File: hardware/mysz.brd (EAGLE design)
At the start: 144.8 x 102.5 mm, 30 parts, among them IC1 LM1117T(H)-3.3, IC2 LM1117T(H)-3.3, U1 NUCLEO-L053R8

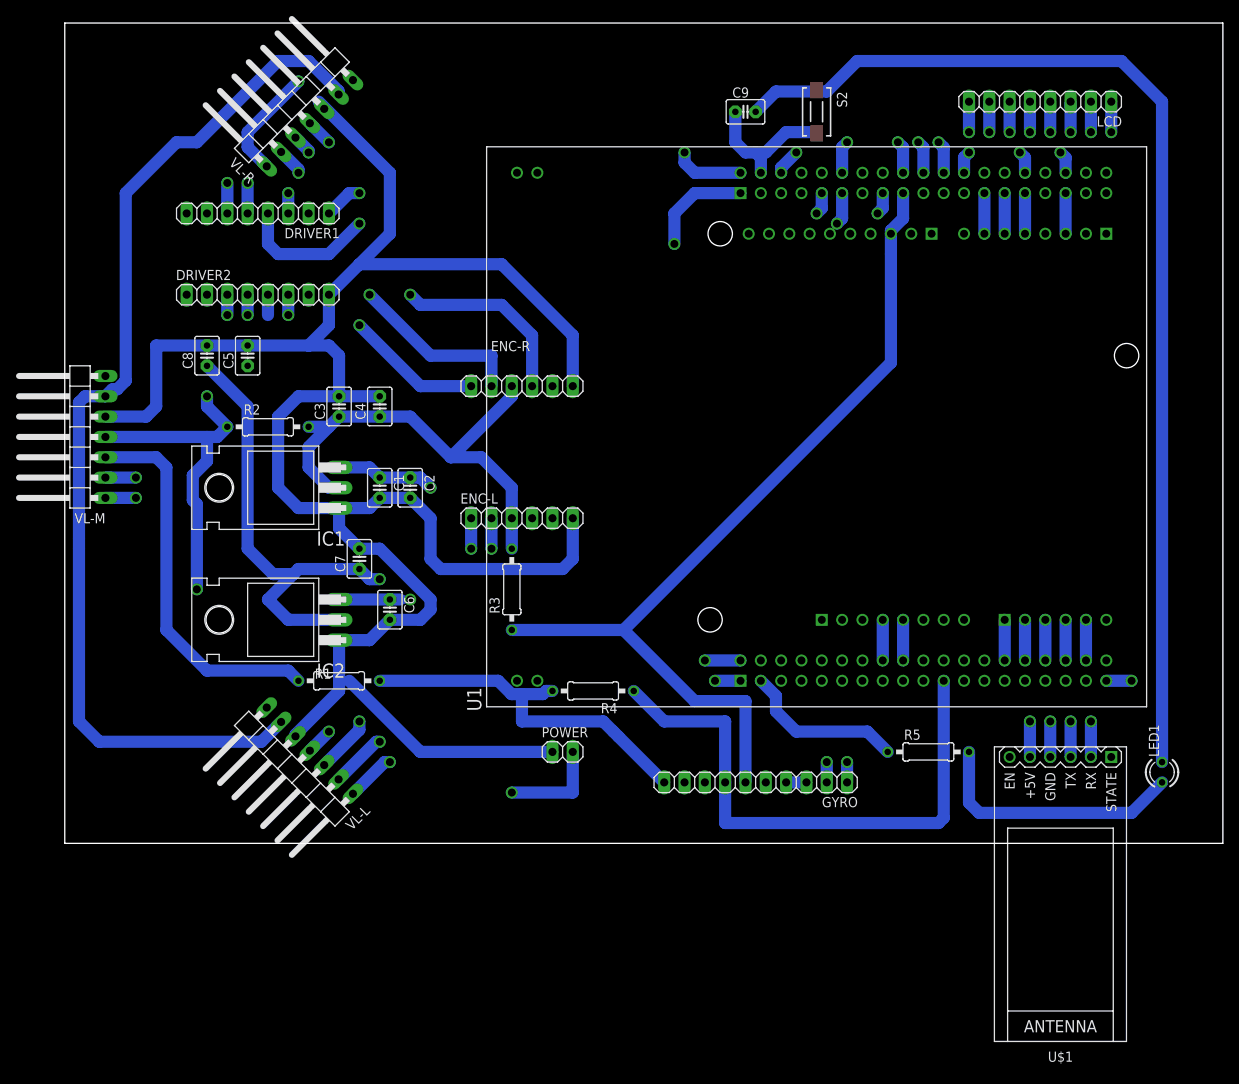
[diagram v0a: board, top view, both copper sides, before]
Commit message: Updated dim.brd
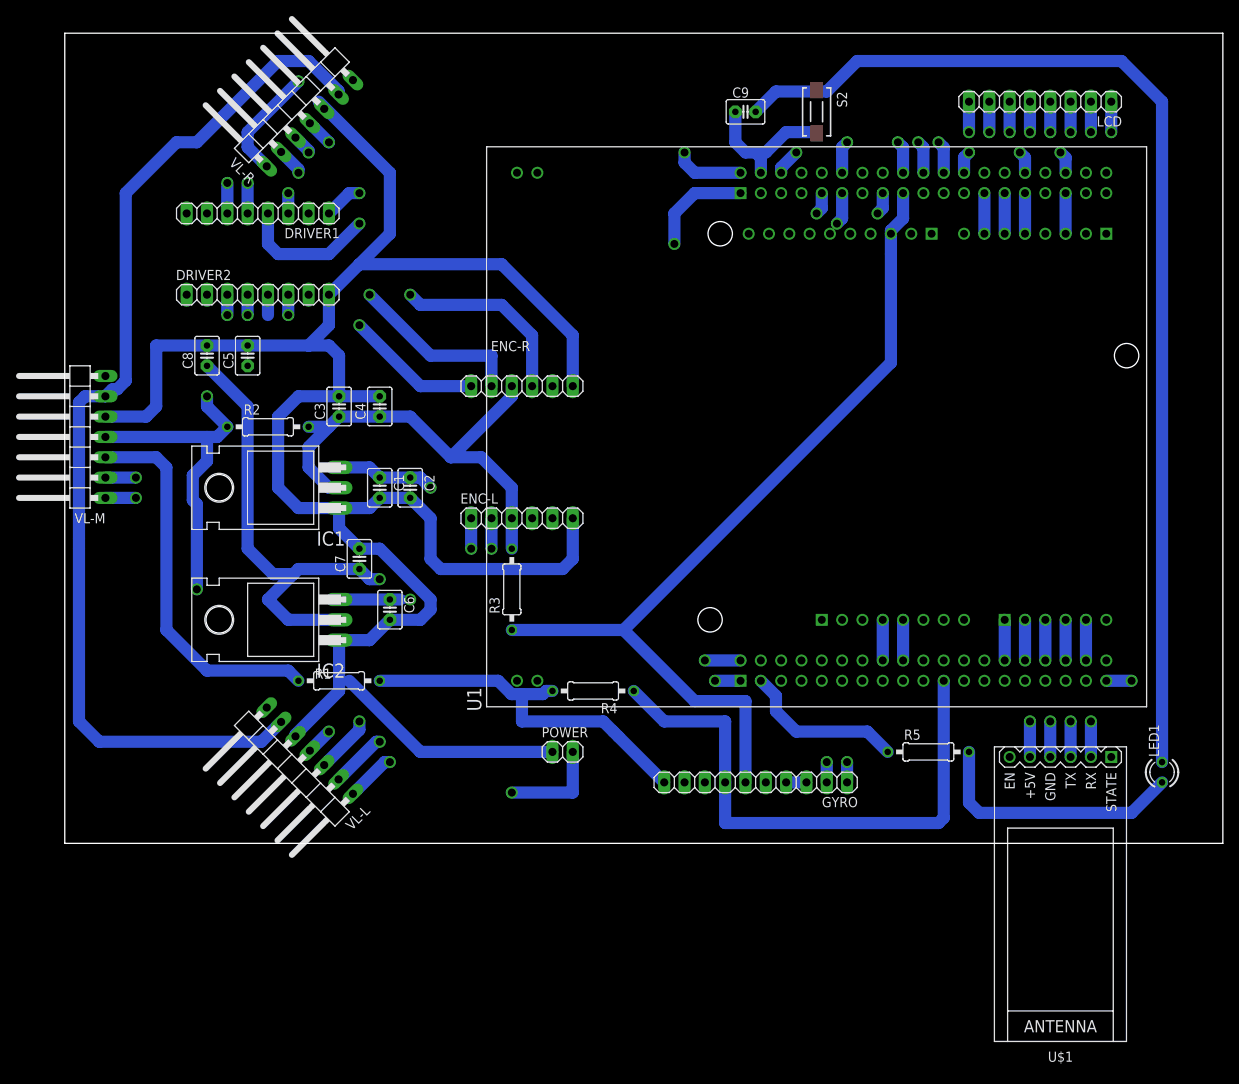
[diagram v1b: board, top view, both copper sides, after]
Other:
- board size 144.8 x 102.5 mm -> 144.8 x 101.3 mm
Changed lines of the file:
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@@
 <plain>
 <wire x1="0" y1="0" x2="144.76" y2="0" width="0" layer="20"/>
-<wire x1="144.76" y1="0" x2="144.76" y2="102.54" width="0" layer="20"/>
-<wire x1="144.76" y1="102.54" x2="0" y2="102.54" width="0" layer="20"/>
-<wire x1="0" y1="102.54" x2="0" y2="0" width="0" layer="20"/>
+<wire x1="144.76" y1="0" x2="144.76" y2="101.27" width="0" layer="20"/>
+<wire x1="144.76" y1="101.27" x2="0" y2="101.27" width="0" layer="20"/>
+<wire x1="0" y1="101.27" x2="0" y2="0" width="0" layer="20"/>
 <dimension x1="-3.81" y1="0" x2="-3.81" y2="100.33" x3="-11.43" y3="50.165" textsize="1.778" layer="1" dtype="horizontal"/>
 <dimension x1="-6.35" y1="0" x2="-6.35" y2="49.53" x3="-6.35" y3="49.53" textsize="1.778" layer="1" dtype="diameter"/>
 <dimension x1="-6.35" y1="49.53" x2="-6.35" y2="100.33" x3="-6.35" y3="100.33" textsize="1.778" layer="1" dtype="diameter"/>
-<dimension x1="64.77" y1="87.63" x2="148.59" y2="87.63" x3="106.68" y3="101.6" textsize="1.778" layer="1"/>
+<dimension x1="0" y1="101.27" x2="144.78" y2="101.6" x3="72.39" y3="111.76" textsize="1.778" layer="1" dtype="horizontal"/>
+<dimension x1="134.62" y1="77.47" x2="53.34" y2="77.47" x3="93.98" y3="105.41" textsize="1.778" layer="1" dtype="horizontal"/>
 </plain>
 <attributes>
